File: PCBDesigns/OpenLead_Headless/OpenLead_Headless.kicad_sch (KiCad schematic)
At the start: 34 parts, among them J1 Conn_01x07_Pin, J2 Battery, J3 Conn_01x07_Pin, J4 Conn_01x01, J5 Conn_01x01, J6 Conn_01x01, Q8 AO3400A MOSFET, SW3 SW_SPDT, U10 LM4040

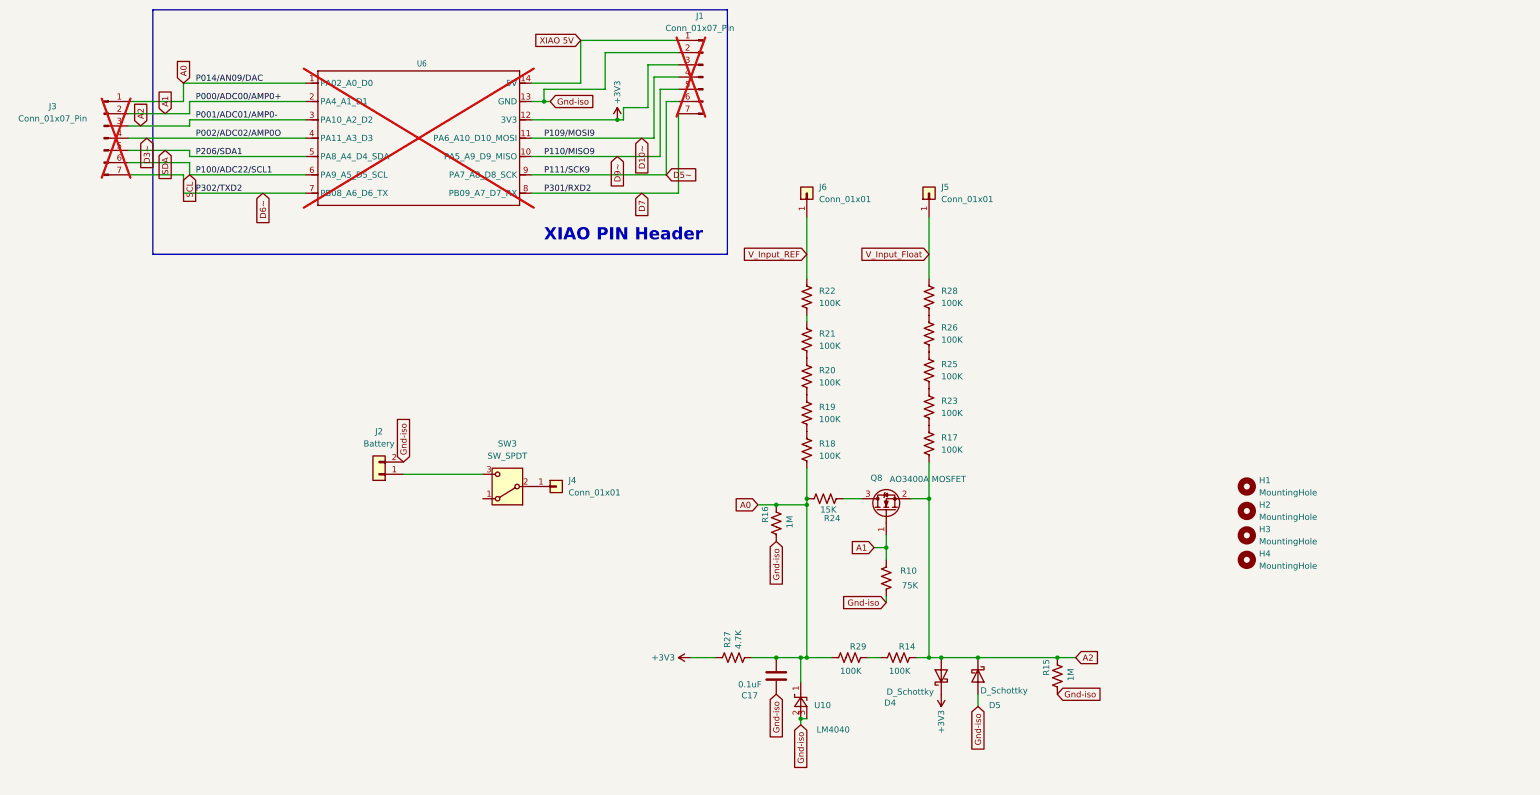
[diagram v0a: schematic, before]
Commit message: Lots of data collection, with some code updates on timings and thresholds.
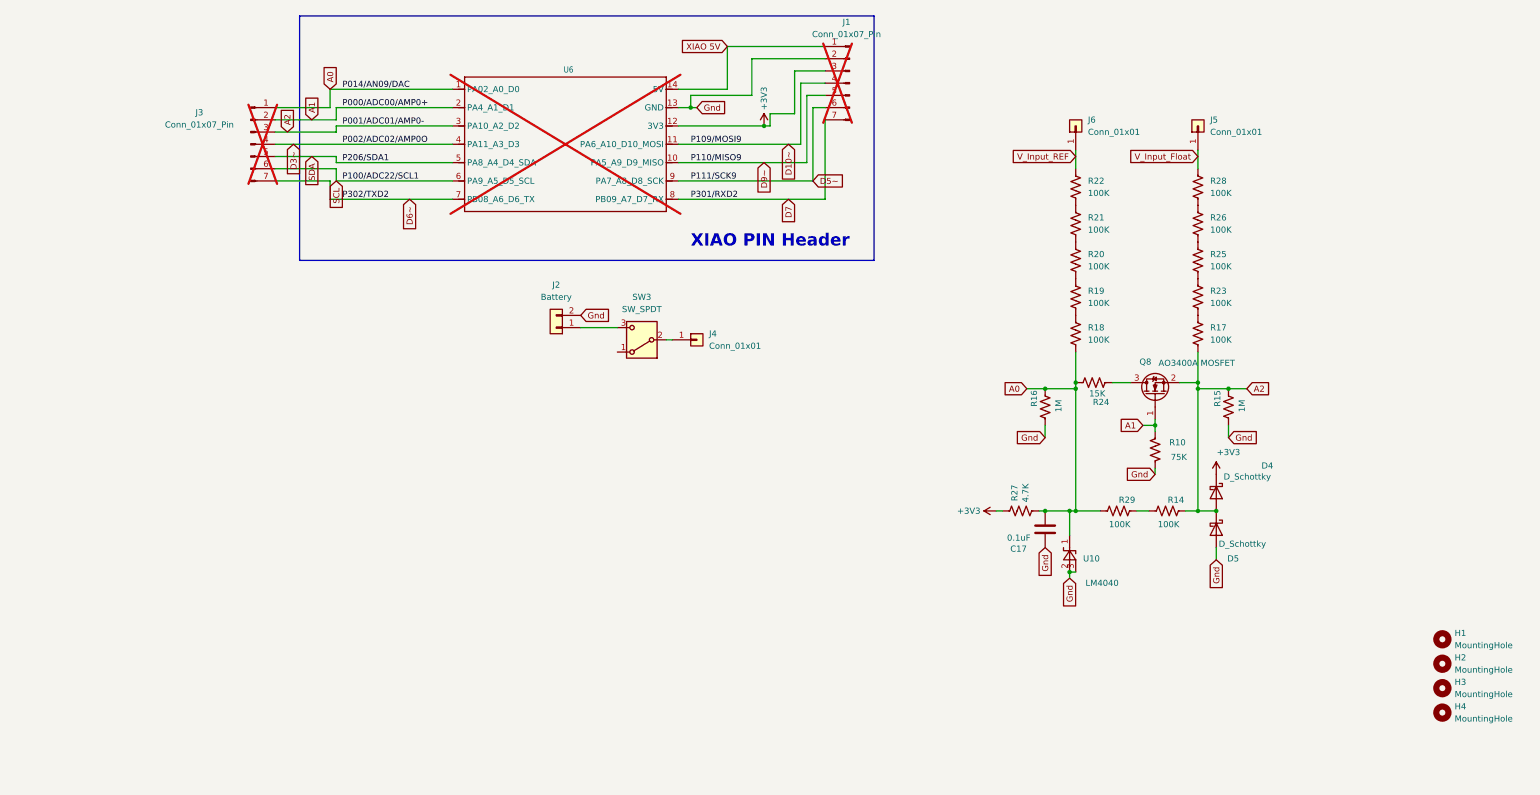
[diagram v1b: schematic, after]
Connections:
- net Gnd-iso renamed Gnd
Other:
- moved on the sheet: C17, D4, D5, H1, H2, H3, H4, J1, J2, J3, J4, J5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
